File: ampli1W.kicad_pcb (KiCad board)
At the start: 2 copper layers, 28 x 35 mm, 17 parts, among them P1 SMA, P2 SMA, P3 CONN_01X01, T1 ADT1.5-1, T2 T4-1-X65, U1 OPA2677

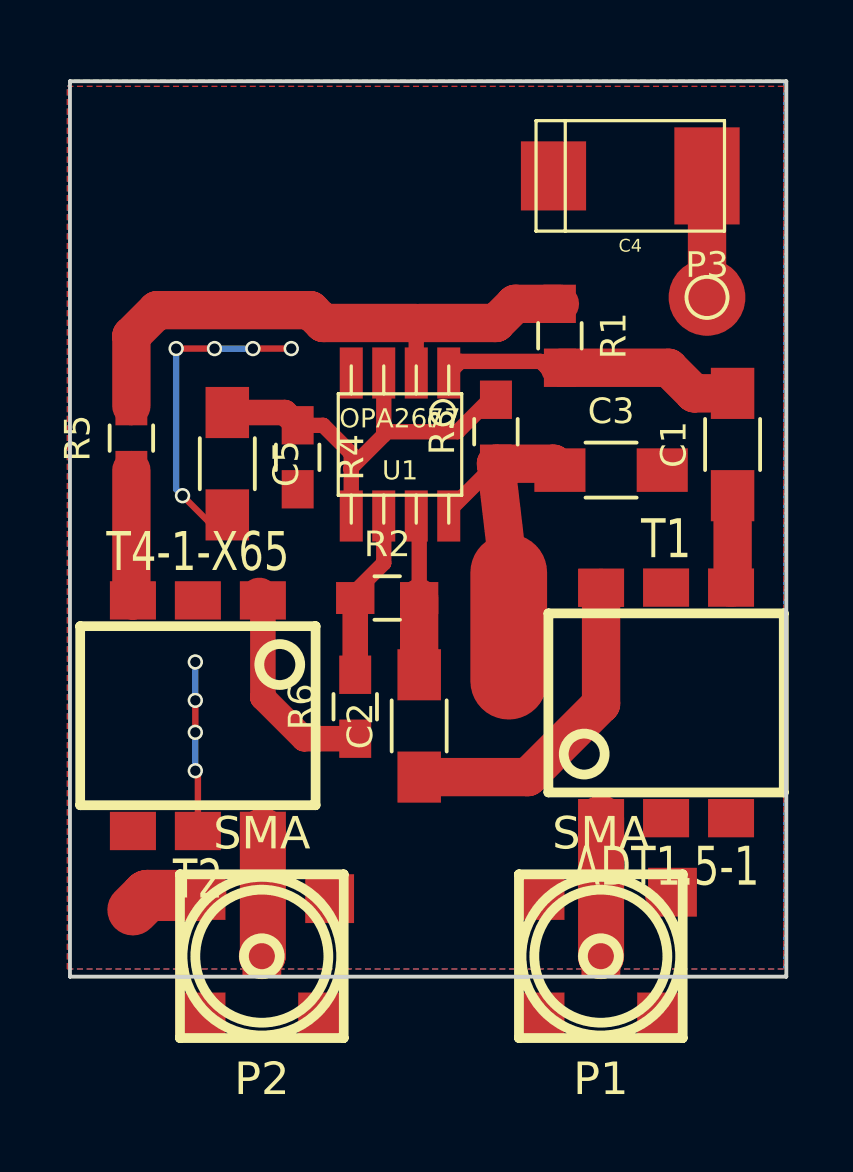
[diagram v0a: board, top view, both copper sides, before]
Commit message: opened and saved with Kicad 8.0.4
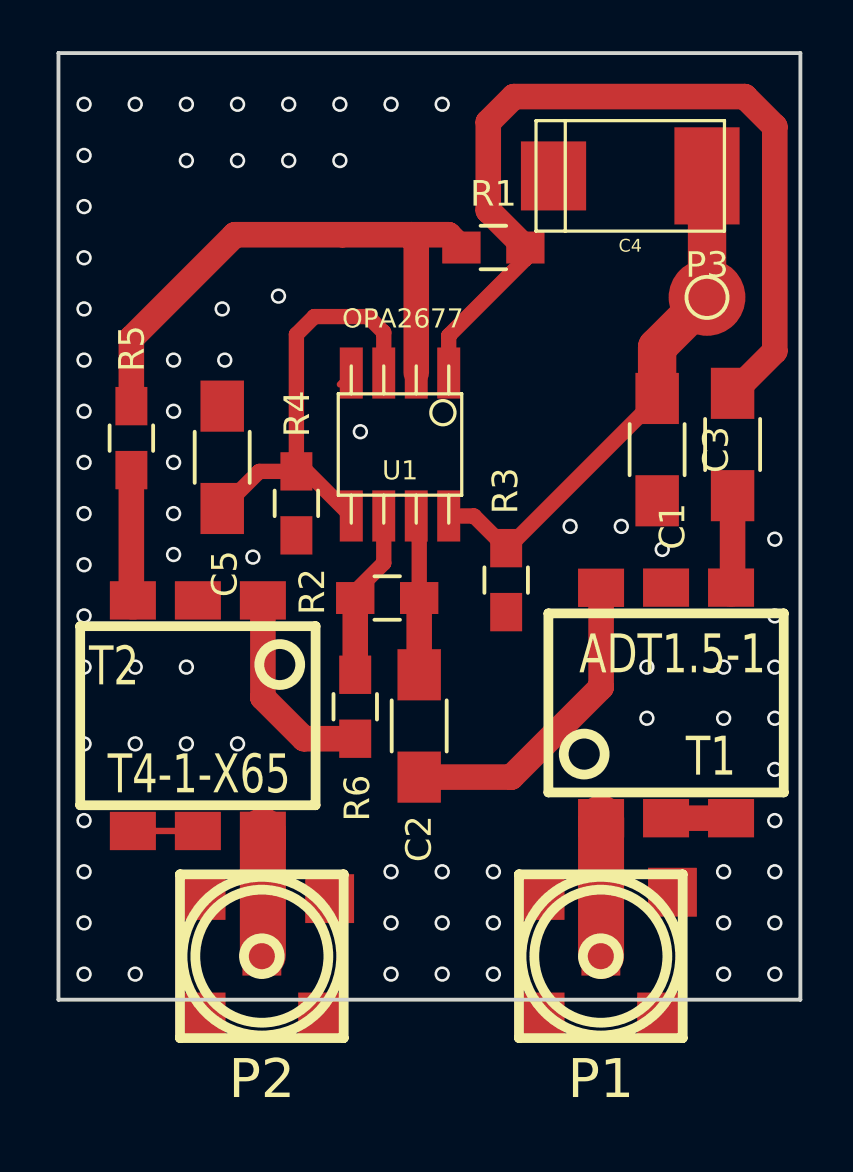
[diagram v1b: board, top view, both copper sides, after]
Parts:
- moved R3 5.81 mm to (157.5, 106.6), turned to -90 degrees
- moved R1 4.32 mm to (157.0, 93.6), turned to 0 degrees
- moved C3 1.97 mm to (163.4, 101.5), turned to -90 degrees
- moved R4 1.80 mm to (149.3, 103.6)
- moved C5 0.32 mm to (146.4, 101.8), turned to 90 degrees
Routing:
- net Net-(C1-Pad2): track 12.1 -> 35.1 mm
- net GND: track 22.8 -> 5.71 mm, vias 9 -> 72
- net +12V: track 18.9 -> 20.8 mm
- net Net-(C5-Pad1): track 17.9 -> 17.0 mm
- net Net-(R1-Pad1): track 22.4 -> 22.9 mm
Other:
- board size 28 x 35 mm -> 29 x 37 mm
- net class Default removed
